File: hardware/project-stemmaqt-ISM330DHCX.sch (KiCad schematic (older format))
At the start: 18 parts, among them J1 SM04B-SRSS-TB(LF)(SN), J2 SM04B-SRSS-TB(LF)(SN), J3 SM04B-SRSS-TB(LF)(SN), U1 TPS7A0218PDBVR, U2 AS7341-DLGT

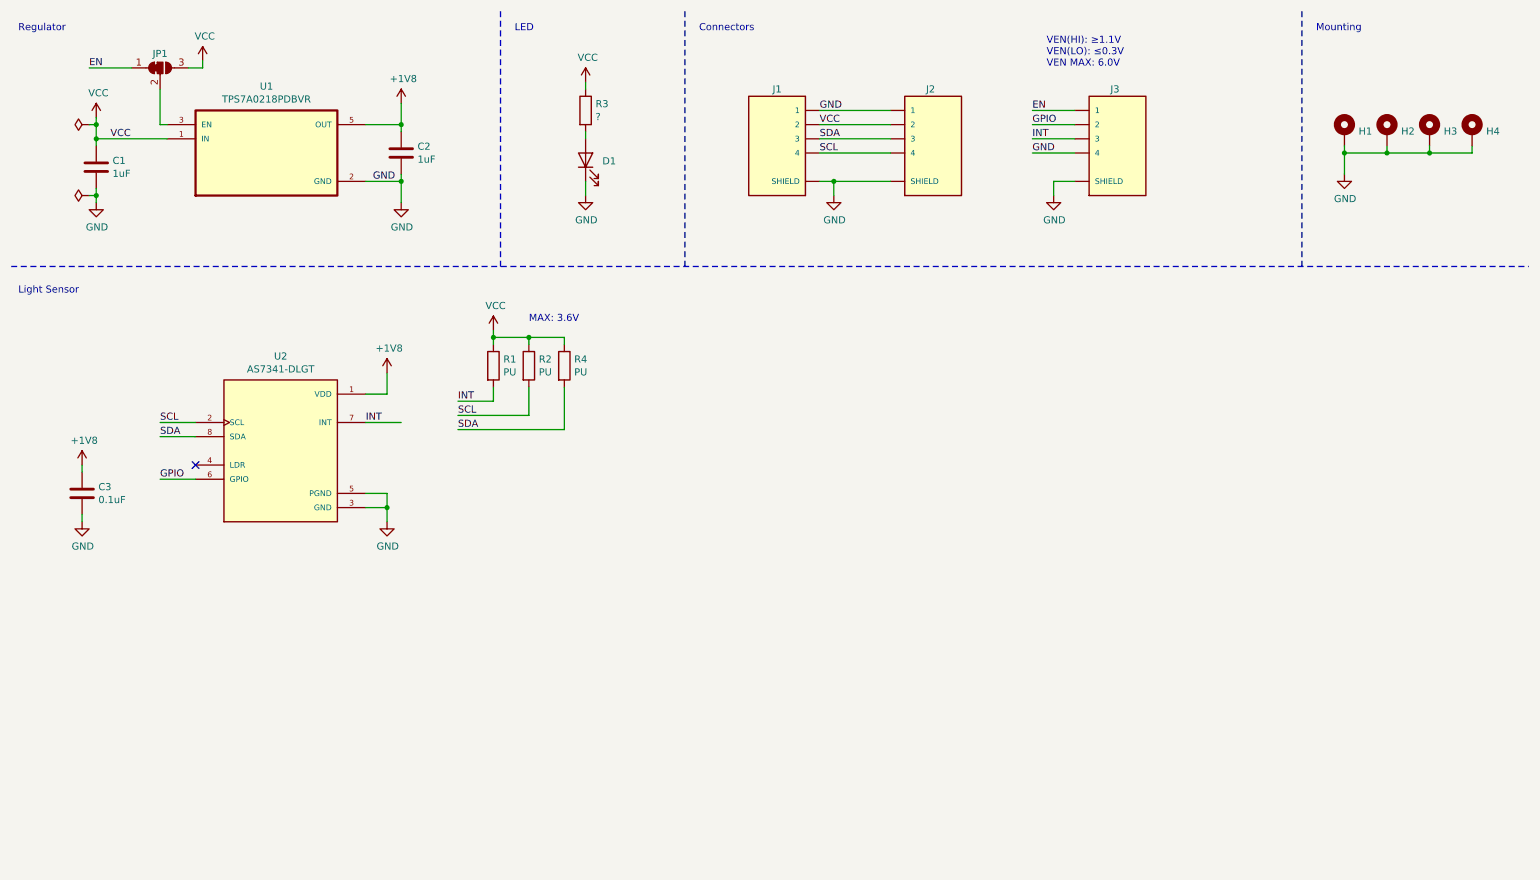
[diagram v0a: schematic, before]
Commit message: First draft
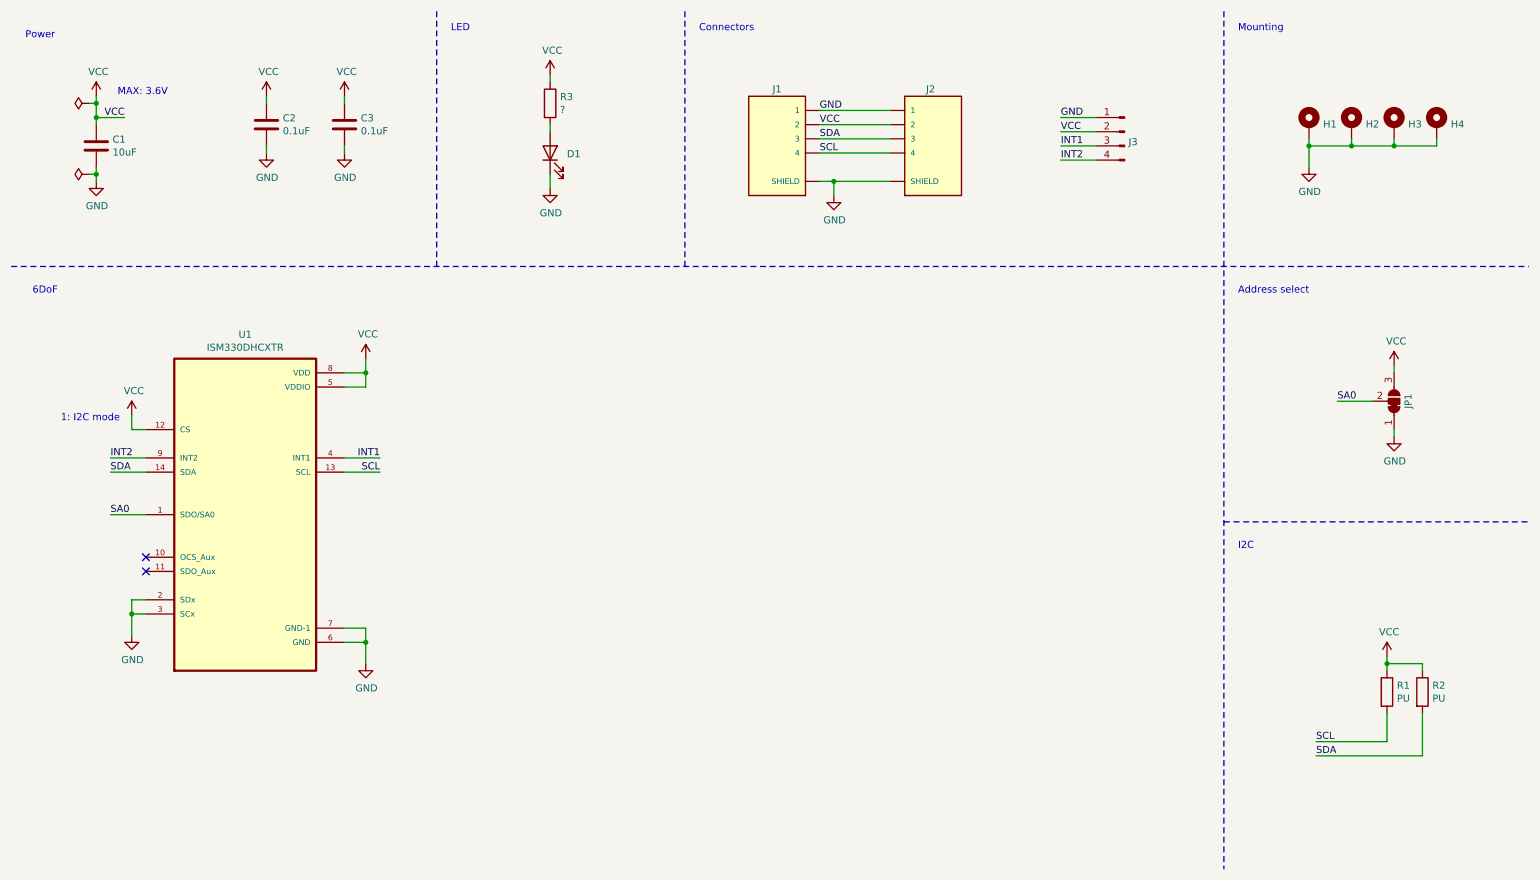
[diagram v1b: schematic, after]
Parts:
- removed J3: SM04B-SRSS-TB(LF)(SN), JST_SM04B-SRSS-TB(LF)(SN), symbol SM04B-SRSS-TB_LF__SN_:SM04B-SRSS-TB(LF)(SN)
- removed R4: PU, Resistor_SMD:R_0603_1608Metric, symbol Device:R
- removed U1: TPS7A0218PDBVR, SOT95P280X145-5N, symbol TPS7A0233PDBVR:TPS7A0233PDBVR
- removed U2: AS7341-DLGT, PSON80P310X200X110-8N, symbol AS7341-DLGT:AS7341-DLGT
- added J3: Conn_01x04_Male, Connector_PinHeader_2.54mm:PinHeader_1x04_P2.54mm_Vertical, symbol Connector:Conn_01x04_Male
- added U1: ISM330DHCXTR, PQFN50P250X300X86-14N, symbol ISM330DHCXTR:ISM330DHCXTR
- C1: value 1uF -> 10uF
- C2: value 1uF -> 0.1uF; footprint Capacitor_SMD:C_0805_2012Metric -> Capacitor_SMD:C_0603_1608Metric
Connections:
- net +1V8 is gone; now on net VCC: C2.1, C3.1
- net EN is gone; now on net GND: JP1.1 (A)
- net INT is gone; now on net SCL: R1.2
- net GND: now also J3.1 (Pin_1), U1.2 (SDx), U1.3 (SCx), U1.6 (GND), U1.7 (GND-1)
- net SCL: now also U1.13 (SCL); no longer R2.2
- net SDA: now also R2.2, U1.14 (SDA)
- net VCC: now also J3.2 (Pin_2), U1.12 (CS), U1.5 (VDDIO), U1.8 (VDD)
- net SA0: now reaches JP1.2 (C)
- net SA0: now also U1.1 (SDO/SA0)
- new net INT1: J3.3 (Pin_3), U1.4 (INT1)
- new net INT2: J3.4 (Pin_4), U1.9 (INT2)
- no-connect marks 1 -> 2
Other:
- note added: "1: I2C mode"
- note added: "6DoF"
- note added: "Address select"
- note added: "I2C"
- note added: "Power"
- note removed: "Light Sensor"
- note removed: "Regulator"
- note removed: "VEN(HI): ≥1.1V\nVEN(LO): ≤0.3V\nVEN MAX: 6.0V"
- moved on the sheet: C1, D1, H1, H2, H3, H4, JP1, R1, R2, R3
